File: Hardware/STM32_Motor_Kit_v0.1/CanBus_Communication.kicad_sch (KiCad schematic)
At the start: 18 parts, among them J3 Conn_01x02_Male, U6 TJA1441BT_0Z

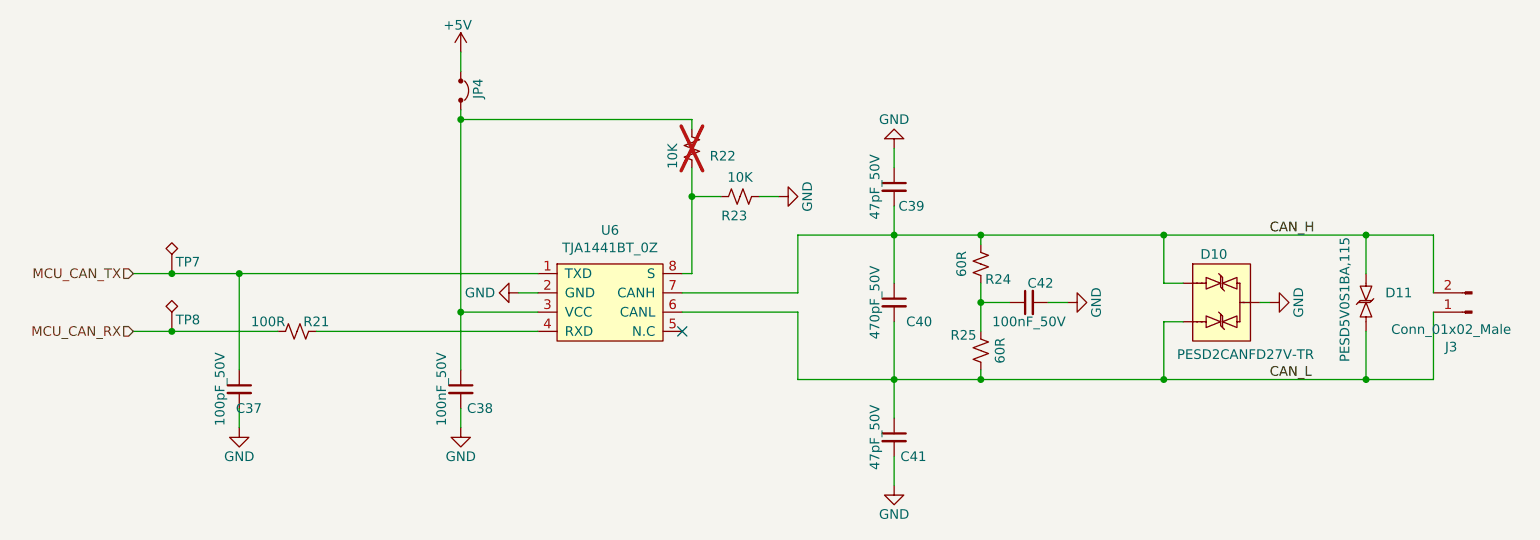
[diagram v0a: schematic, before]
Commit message: 12.01.2025
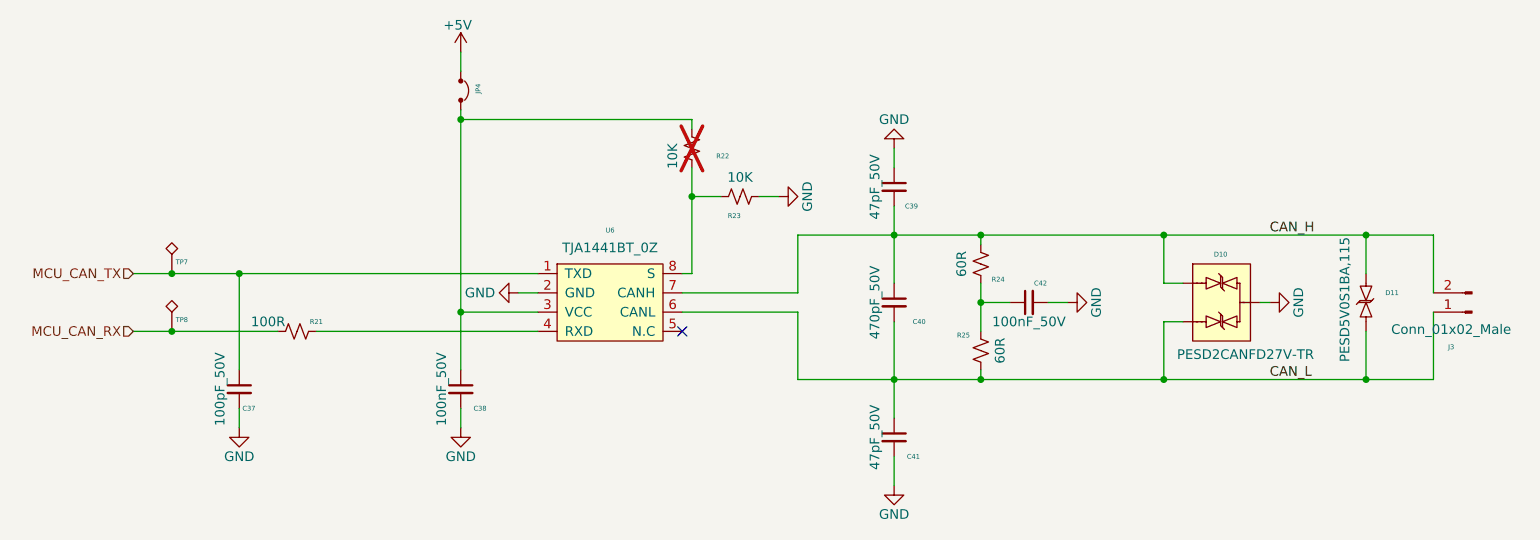
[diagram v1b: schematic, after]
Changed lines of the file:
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@@
 			(effects
 				(font
-					(size 1.27 1.27)
+					(face "Arial")
+					(size 0.635 0.635)
 				)
 				(hide yes)
@@
 			(effects
 				(font
-					(size 1.27 1.27)
+					(face "Arial")
+					(size 0.635 0.635)
 				)
 				(justify right)
@@
 			(effects
 				(font
-					(size 1.27 1.27)
+					(face "Arial")
+					(size 0.635 0.635)
 				)
 				(hide yes)
@@
 			(effects
 				(font
-					(size 1.27 1.27)
+					(face "Arial")
+					(size 0.635 0.635)
 				)
 				(hide yes)
@@
 			(effects
 				(font
-					(size 1.27 1.27)
+					(face "Arial")
+					(size 0.635 0.635)
 				)
 				(justify left)
@@
 			(effects
 				(font
-					(size 1.27 1.27)
+					(face "Arial")
+					(size 0.635 0.635)
 				)
 				(hide yes)
@@
 			(effects
 				(font
-					(size 1.27 1.27)
+					(face "Arial")
+					(size 0.635 0.635)
 				)
 			)
@@
 			(effects
 				(font
-					(size 1.27 1.27)
+					(face "Arial")
+					(size 0.635 0.635)
 				)
 				(justify left)
@@
 			(effects
 				(font
-					(size 1.27 1.27)
+					(face "Arial")
+					(size 0.635 0.635)
 				)
 				(hide yes)
@@
 			(effects
 				(font
-					(size 1.27 1.27)
+					(face "Arial")
+					(size 0.635 0.635)
 				)
 			)
@@
 			(effects
 				(font
-					(size 1.27 1.27)
+					(face "Arial")
+					(size 0.635 0.635)
 				)
 			)
@@
 			(effects
 				(font
-					(size 1.27 1.27)
+					(face "Arial")
+					(size 0.635 0.635)
 				)
 				(hide yes)
@@
 			(effects
 				(font
-					(size 1.27 1.27)
+					(face "Arial")
+					(size 0.635 0.635)
 				)
 			)
@@
 			(effects
 				(font
-					(size 1.27 1.27)
+					(face "Arial")
+					(size 0.635 0.635)
 				)
 				(justify left)
@@
 			(effects
 				(font
-					(size 1.27 1.27)
+					(face "Arial")
+					(size 0.635 0.635)
 				)
 			)
@@
 			(effects
 				(font
-					(size 1.27 1.27)
+					(face "Arial")
+					(size 0.635 0.635)
 				)
 			)
@@
 			(effects
 				(font
-					(size 1.27 1.27)
+					(face "Arial")
+					(size 0.635 0.635)
 				)
 			)
@@
 			(effects
 				(font
-					(size 1.27 1.27)
+					(face "Arial")
+					(size 0.635 0.635)
 				)
 			)
@@
 			(effects
 				(font
-					(size 1.27 1.27)
+					(face "Arial")
+					(size 0.635 0.635)
 				)
 			)
@@
 			(effects
 				(font
-					(size 1.27 1.27)
+					(face "Arial")
+					(size 0.635 0.635)
 				)
 			)
@@
 			(effects
 				(font
-					(size 1.27 1.27)
+					(face "Arial")
+					(size 0.635 0.635)
 				)
 			)
@@
 			(effects
 				(font
-					(size 1.27 1.27)
+					(face "Arial")
+					(size 0.635 0.635)
 				)
 			)
@@
 			(effects
 				(font
-					(size 1.27 1.27)
+					(face "Arial")
+					(size 0.635 0.635)
 				)
 				(hide yes)
@@
 			(effects
 				(font
-					(size 1.27 1.27)
+					(face "Arial")
+					(size 0.635 0.635)
 				)
 				(hide yes)
@@
 			(effects
 				(font
-					(size 1.27 1.27)
+					(face "Arial")
+					(size 0.635 0.635)
 				)
 			)
@@
 			(effects
 				(font
-					(size 1.27 1.27)
+					(face "Arial")
+					(size 0.635 0.635)
 				)
 				(hide yes)
@@
 			(effects
 				(font
-					(size 1.27 1.27)
-				)
-			)
+					(face "Arial")
+					(size 0.635 0.635)
+				)
+			)
